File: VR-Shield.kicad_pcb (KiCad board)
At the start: 2 copper layers, 21 parts, among them Q1 IRF7404, Q2 BC847, U1 ESP32 WROOM32 Devkit, U2 MCP73831-2-OT

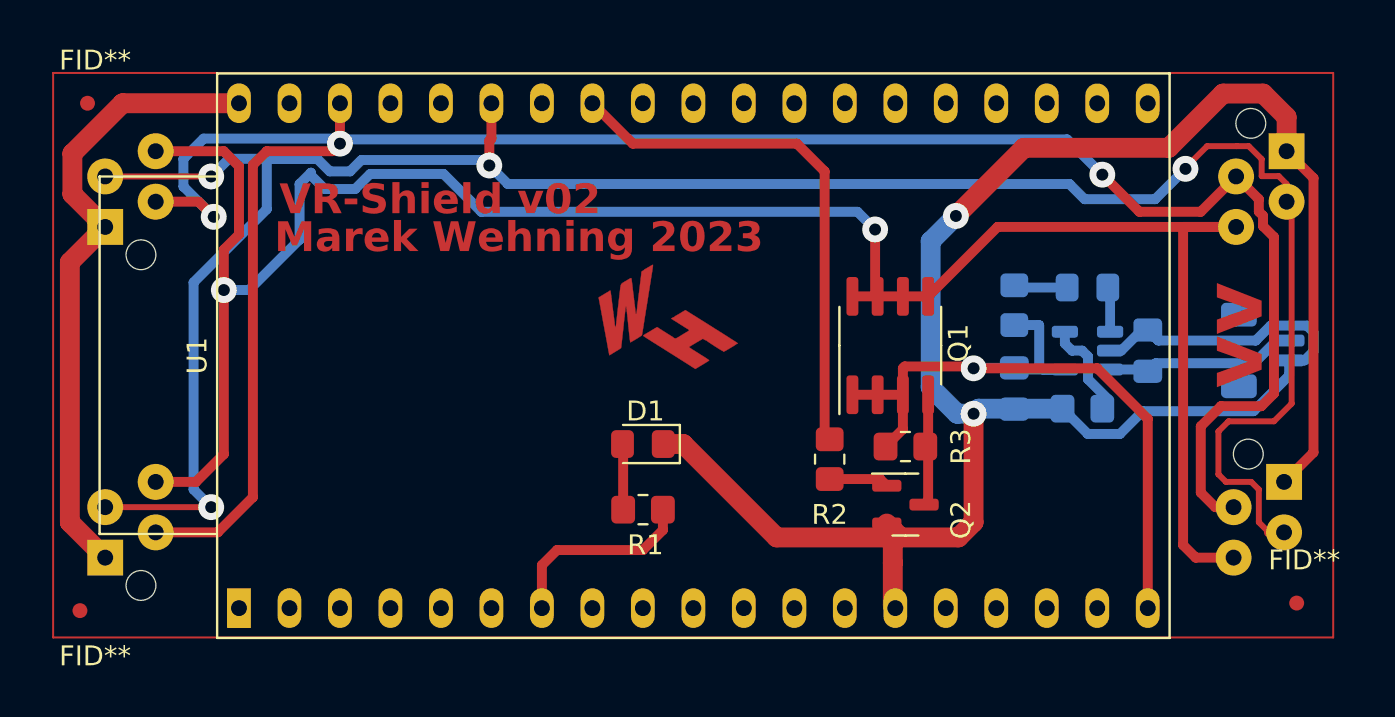
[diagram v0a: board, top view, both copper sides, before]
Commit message: t V03!!!!
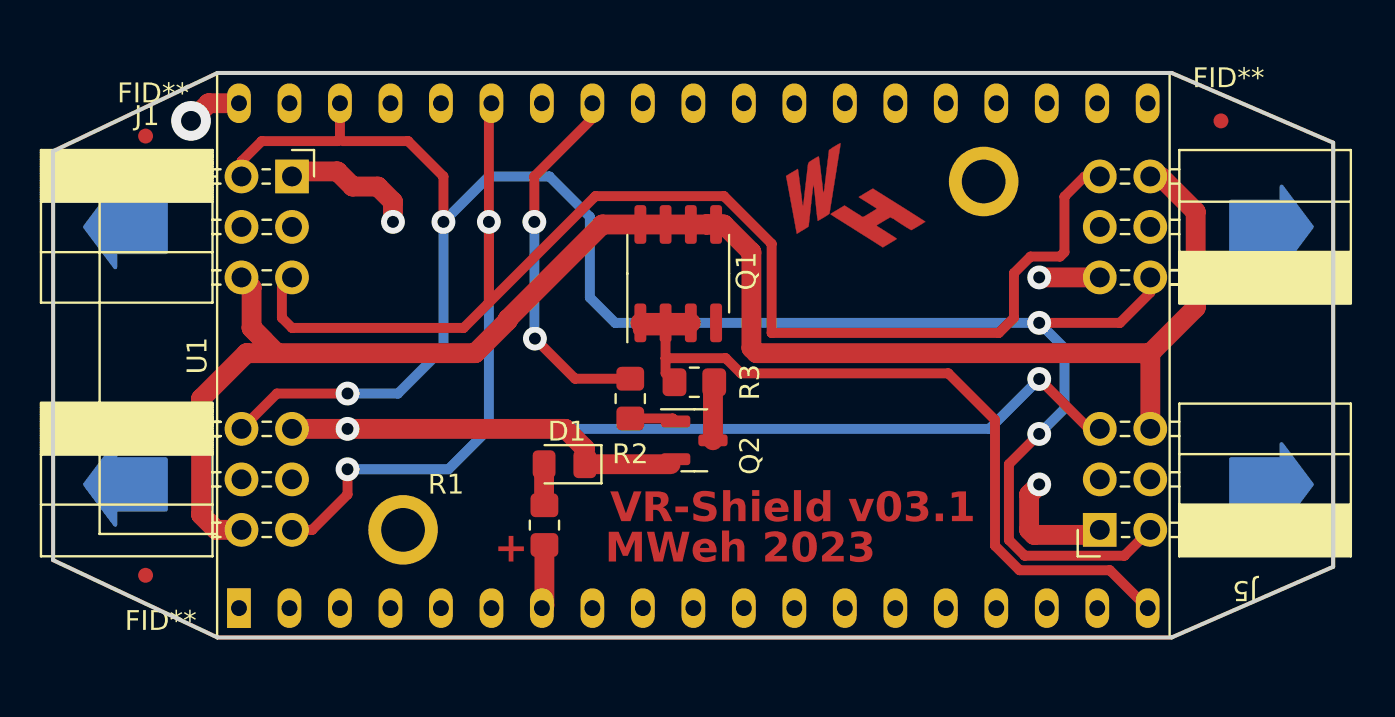
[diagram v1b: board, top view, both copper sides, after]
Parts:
- removed BT1: Battery_Cell, Connector_JST:JST_SH_BM02B-SRSS-TB_1x02-1MP_P1.00mm_Vertical
- removed C1: C, Capacitor_SMD:C_0805_2012Metric_Pad1.18x1.45mm_HandSolder
- removed C2: 4,7u, Capacitor_SMD:C_0805_2012Metric_Pad1.18x1.45mm_HandSolder
- removed D2: GREEN, LED_SMD:LED_0805_2012Metric_Pad1.15x1.40mm_HandSolder
- removed P1, P2, P3, P4: ~, Custom:TE_Micro-MaTch_215079-4_2x02_P1.27mm_Vertical
- removed R4: 10k, Resistor_SMD:R_0805_2012Metric_Pad1.20x1.40mm_HandSolder
- removed R5: 470, Resistor_SMD:R_0805_2012Metric_Pad1.20x1.40mm_HandSolder
- removed U2: MCP73831-2-OT, Package_TO_SOT_SMD:SOT-23-5
- added ?: , , F.Cu at (60.7, 19.6)
- added J1: Double I2C Socket, Custom:Custom Socket I2C, F.Cu at (18.6, 28.2)
- added J5: Double I2C Socket, Custom:Custom Socket I2C, F.Cu at (73.8, 28.2)
- added REF**: MountingHole_2.2mm_M2_ISO7380_Pad, MountingHole:MountingHole_2.2mm_M2_ISO7380_Pad, F.Cu at (31.5, 37.1)
- moved FID** 24.6 mm to (72.6, 16.5)
- moved Q1 11.3 mm to (45.3, 24.2)
- moved R3 11.1 mm to (46.1, 29.7)
- moved Q2 11.1 mm to (46.1, 32.6)
- moved R2 10.5 mm to (42.9, 30.5)
- moved R1 5.02 mm to (38.6, 36.8), turned to 90 degrees
- moved D1 4.07 mm to (39.6, 33.8)
- moved FID** 3.75 mm to (18.5, 39.4)
- moved FID** 3.36 mm to (18.5, 17.3)
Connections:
- net Net-(P1-VCC) renamed /VCC
- U1 pad 33: Net-(P1-SDA) -> /SDA
- U1 pad 36: Net-(P1-SCL) -> /SCL
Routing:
- net /SDA: track 0.00 -> 124.1 mm, vias 0 -> 3
- net Net-(P1-SDA): track 117.1 -> 0.00 mm, vias 4 -> 0
- net Net-(P1-SCL): track 113.3 -> 0.00 mm, vias 3 -> 0
- net GND: track 143.3 -> 39.2 mm, vias 2 -> 5
- net /SCL: track 0.00 -> 98.2 mm, vias 0 -> 4
- net /VCC: track 107.7 -> 86.1 mm, vias 2 -> 0
- net Net-(BT1-+): track 9.68 -> 0.00 mm
- net Net-(U1-GPIO19): track 26.7 -> 18.7 mm, vias 0 -> 2
- net /LED: track 10.0 -> 3.23 mm
- net Net-(U2-PROG): track 5.16 -> 0.00 mm
- net Net-(Q1-G): track 5.73 -> 2.95 mm
- net Net-(D2-A): track 2.70 -> 0.00 mm
- net Net-(D2-K): track 2.27 -> 0.00 mm
- net /5V: track 39.1 -> 41.1 mm, vias 1 -> 0
- net Net-(D1-A): track 3.32 -> 2.07 mm
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- added copper zone on B.Cu, net GND
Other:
- board outline added: 64.4 x 28.4 mm
- board text added: "+"
- board text added: "MWeh 2023"
- board text added: "VR-Shield v03.1"
- board text removed: "Marek Wehning 2023"
- board text removed: "VR-Shield v02"
- board text removed: "vv"
